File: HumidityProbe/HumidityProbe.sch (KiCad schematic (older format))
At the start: 10 parts

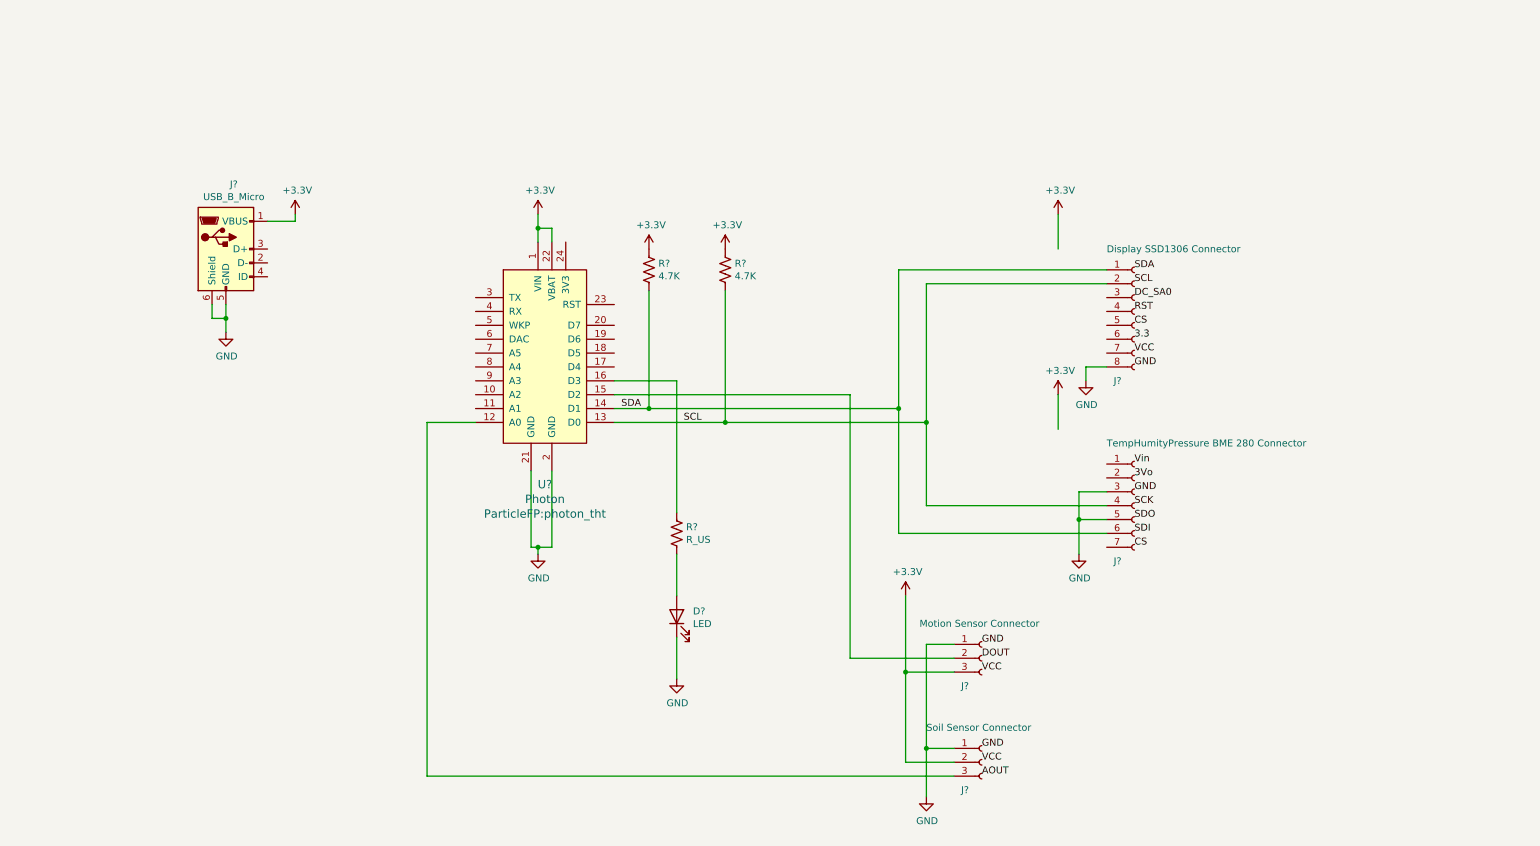
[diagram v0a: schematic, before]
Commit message: added
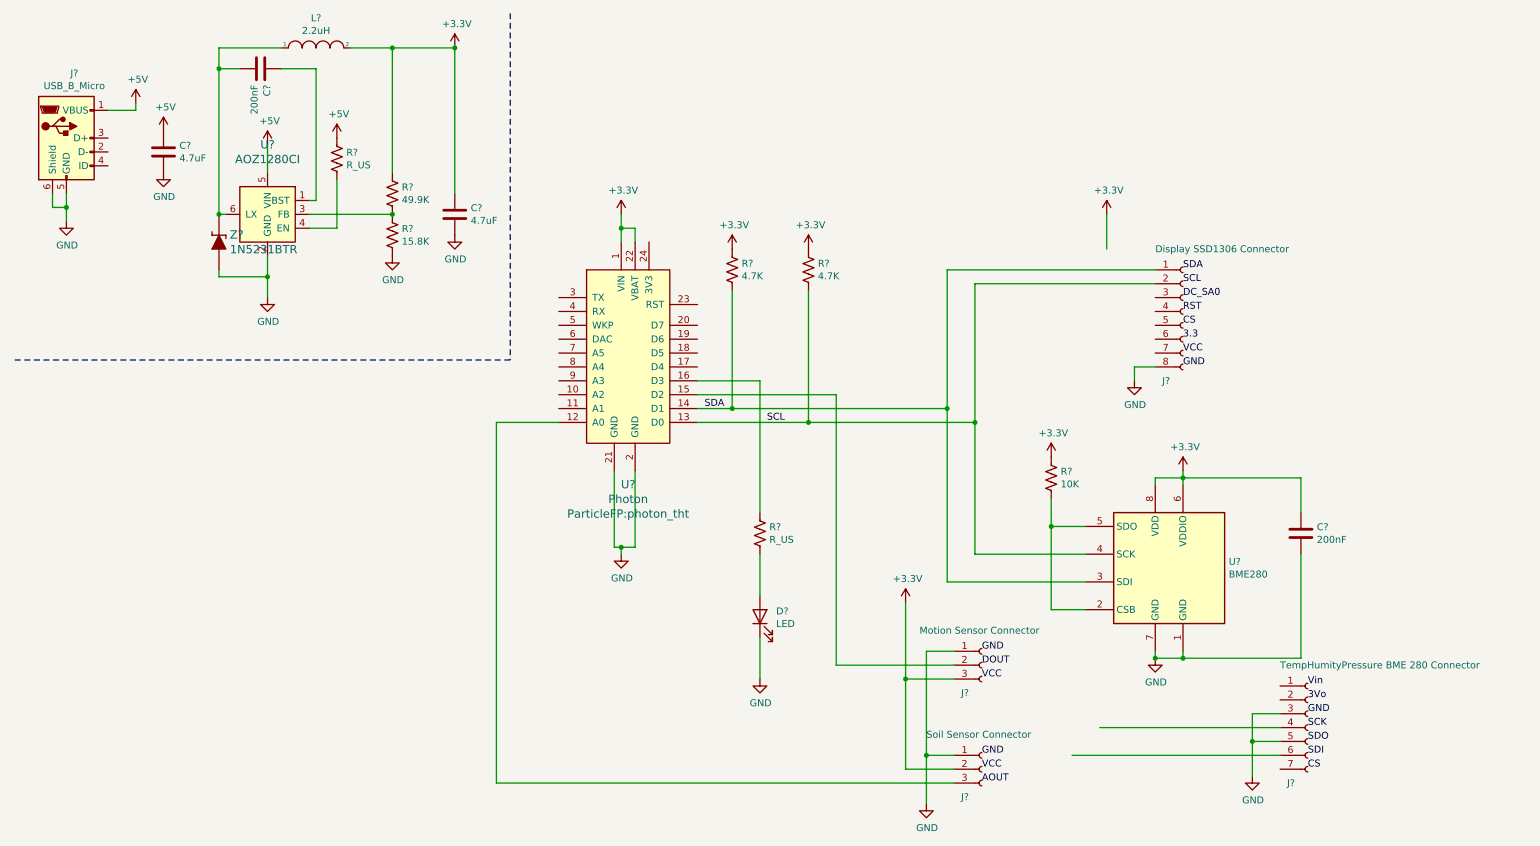
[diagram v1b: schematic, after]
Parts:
- added C? (x2): 200nF, Capacitor_THT:C_Disc_D8.0mm_W5.0mm_P7.50mm, symbol Device:C
- added C? (x2): 4.7uF, Capacitor_THT:C_Disc_D8.0mm_W5.0mm_P7.50mm, symbol Device:C
- added L?: 2.2uH, symbol pspice:INDUCTOR
- added R?: 10K, Resistor_THT:R_Axial_DIN0204_L3.6mm_D1.6mm_P7.62mm_Horizontal, symbol Device:R_US
- added R?: 15.8K, symbol Device:R_US
- added R?: 49.9K, symbol Device:R_US
- added R?: R_US, symbol Device:R_US
- added U?: BME280, Package_LGA:Bosch_LGA-8_2.5x2.5mm_P0.65mm_ClockwisePinNumbering, symbol Sensor:BME280
- added U?: AOZ1280CI, digikey-footprints:SOT-23-6, symbol dk_PMIC-Voltage-Regulators-DC-DC-Switching-Regulators:AOZ1280CI
- added Z?: 1N5231BTR, digikey-footprints:DO-35, symbol dk_Diodes-Zener-Single:1N5231BTR
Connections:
- net labels added: +5V
- wire segments 55 -> 91
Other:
- moved on the sheet: D?, J?, R?, U?
